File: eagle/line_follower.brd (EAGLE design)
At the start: 100 x 80 mm, 41 parts, among them IC1 A4950, IC2 A4950, IC3 MC78M05 (??), J1 2S - 4S LiPo, J2 22-27-2031-03, J3 22-27-2061-06, J4 22-27-2061-06, Q1 ALS-PT19-315C/L177/TR8, Q2 ALS-PT19-315C/L177/TR8, Q3 ALS-PT19-315C/L177/TR8, Q4 ALS-PT19-315C/L177/TR8, Q5 ALS-PT19-315C/L177/TR8, SW1 12MM_BUTTON, X1 ESP32DEVKITV1, X2 MPU6050_BREAKOUT

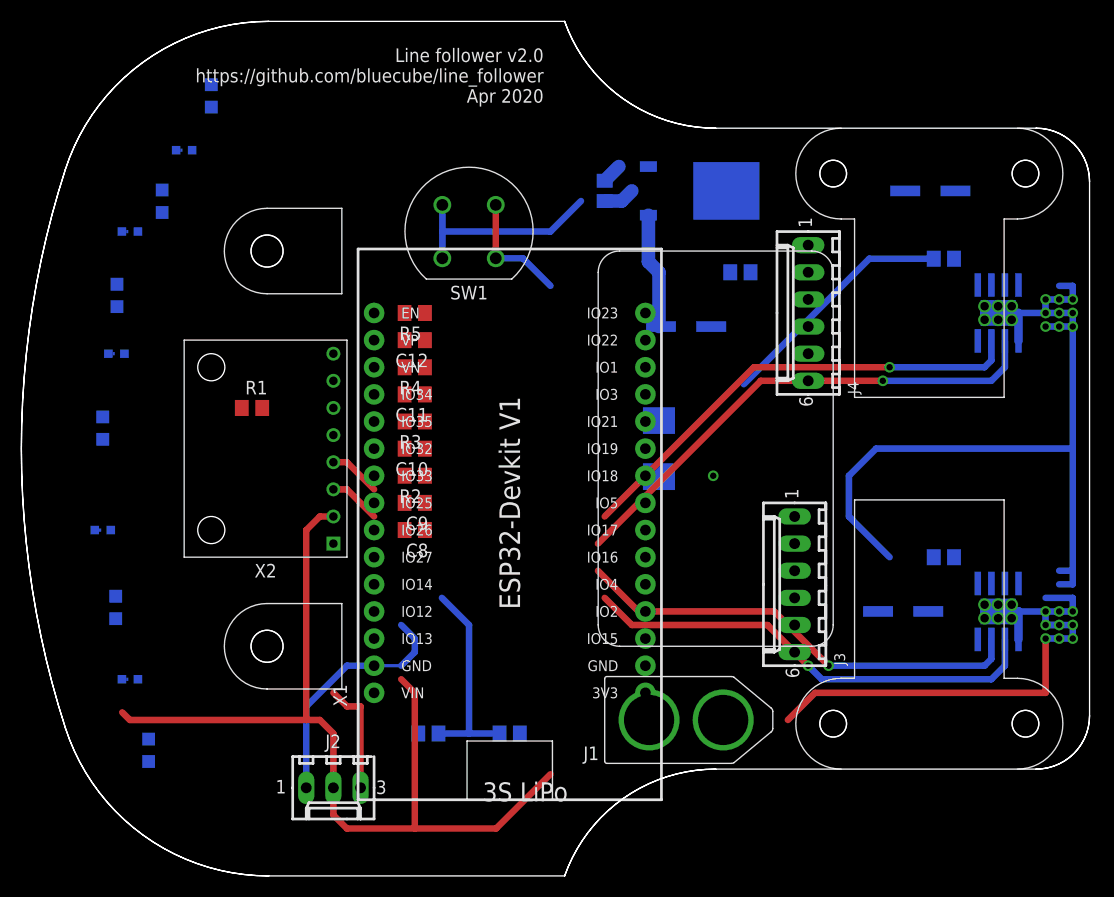
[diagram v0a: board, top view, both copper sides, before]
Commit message: Rough layout of the new board
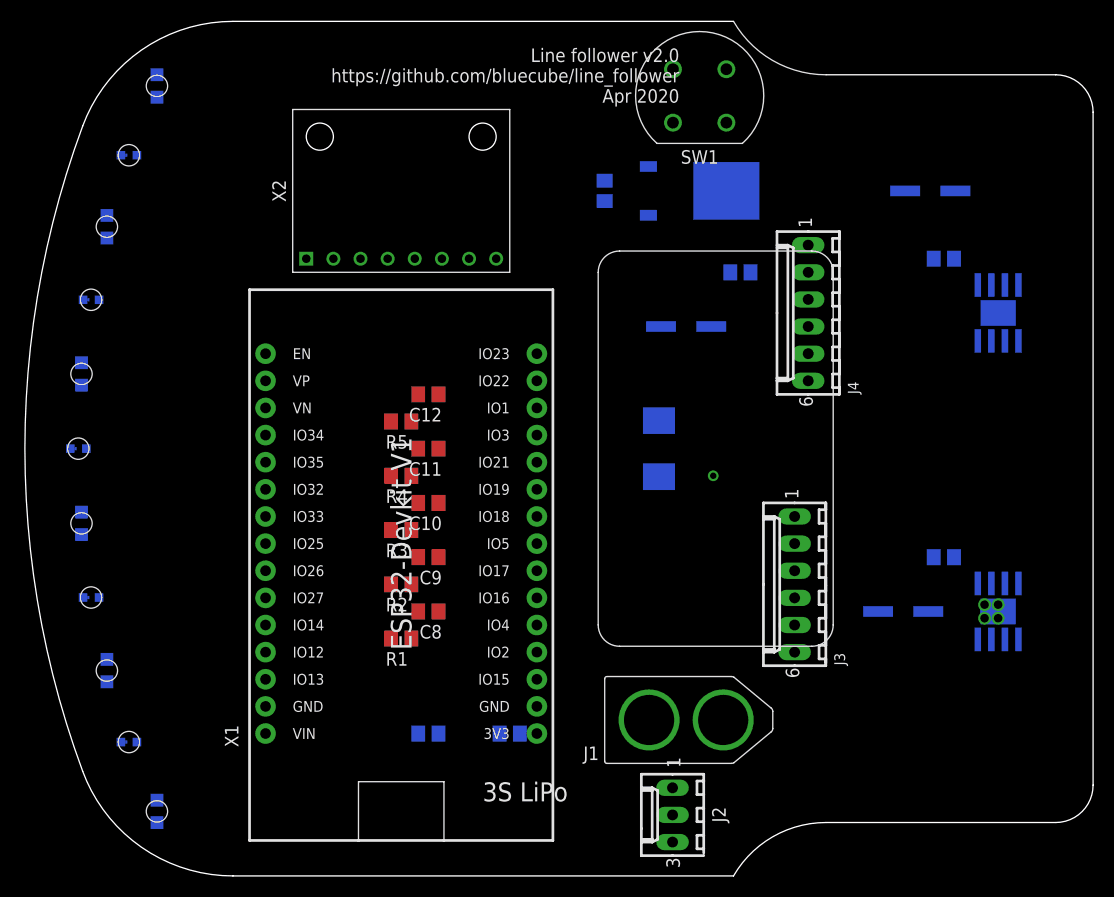
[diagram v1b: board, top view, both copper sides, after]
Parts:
- moved J2 31.9 mm to (61.0, 5.08), turned to 90 degrees
- moved X2 27.3 mm to (35.6, 63.5), turned to 90 degrees
- moved R1 25.7 mm to (35.6, 21.6), turned to 180 degrees
- moved SW1 25.0 mm to (63.5, 72.4)
- moved X1 10.9 mm to (35.6, 30.5)
- moved R4 10.2 mm to (35.6, 36.8)
- moved R5 10.2 mm to (35.6, 41.9)
- moved R2 10.2 mm to (35.6, 26.7)
- moved R3 10.2 mm to (35.6, 31.8)
- moved Q3 9.58 mm to (5.33, 39.4)
- moved LED3 9.13 mm to (5.63, 32.4)
- moved LED4 8.07 mm to (5.63, 46.4)
- moved C8 7.73 mm to (38.1, 24.1)
- moved Q2 7.35 mm to (6.52, 53.3)
- moved Q4 6.41 mm to (6.52, 25.4)
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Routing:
- net GND: track 274.9 -> 4.71 mm, vias 30 -> 4
- net MOTOR1A: track 47.4 -> 0.00 mm, vias 1 -> 0
- net MOTOR1B: track 44.1 -> 0.00 mm, vias 1 -> 0
- net MOTOR0B: track 43.6 -> 0.00 mm, vias 1 -> 0
- net MOTOR0A: track 42.6 -> 0.00 mm, vias 1 -> 0
- net RANGE: track 23.0 -> 0.00 mm
- net BAT_SENSE: track 19.5 -> 0.00 mm
- net BUTTON: track 11.2 -> 0.00 mm
- net N$7: track 10.8 -> 0.00 mm
- net +5V: track 10.7 -> 0.00 mm
- net SDA: track 4.86 -> 0.00 mm
- net SCL: track 4.86 -> 0.00 mm
- net N$6: track 1.88 -> 0.00 mm
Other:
- outline, holes or cut-outs redrawn
